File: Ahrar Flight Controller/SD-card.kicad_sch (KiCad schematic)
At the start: 16 parts, among them J4 1040310811

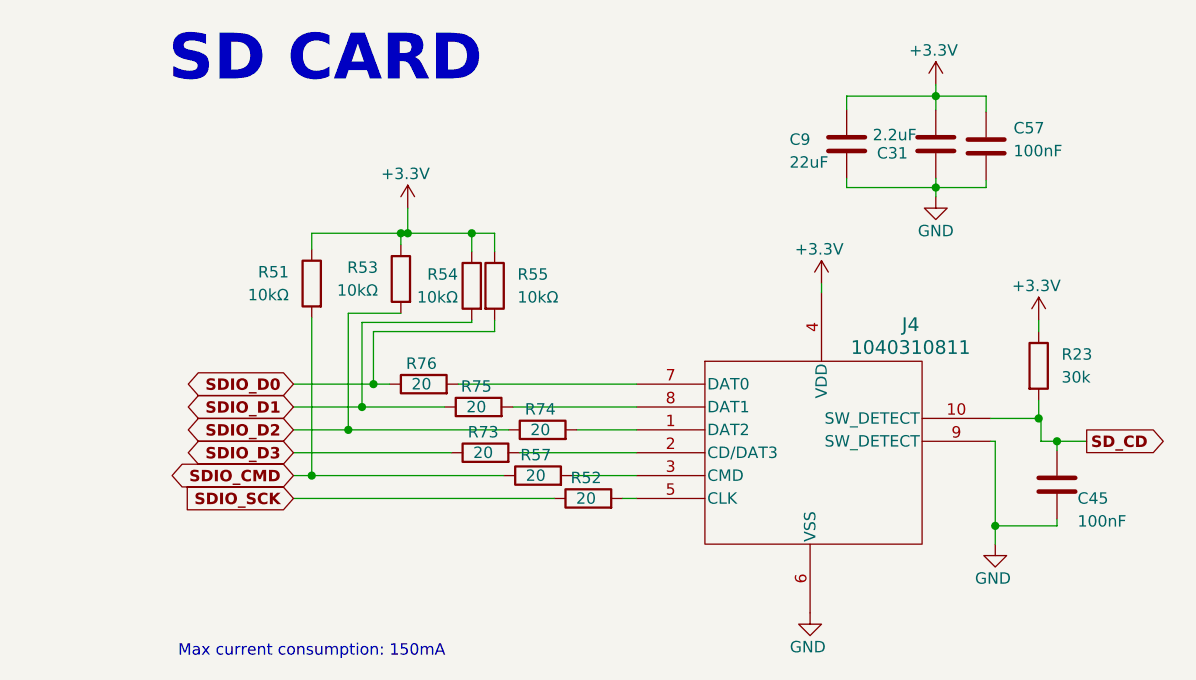
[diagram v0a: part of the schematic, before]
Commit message: .
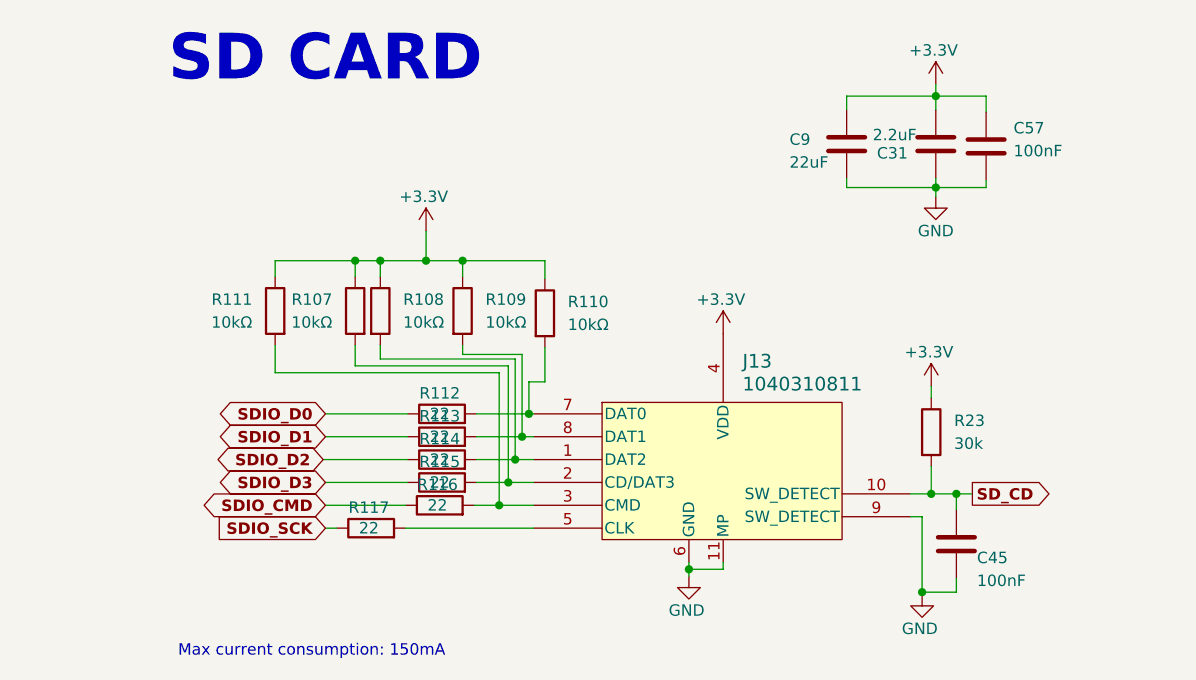
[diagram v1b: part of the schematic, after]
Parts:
- removed J4: 1040310811, Molex 1040310811:104031-0811_MOL, symbol 2026-07-10_16-12-29:1040310811
- removed R51, R53, R54, R55: 10kΩ, Resistor_SMD:R_0402_1005Metric, symbol Device:R
- removed R52, R57, R73, R74, R75, R76: 20, Resistor_SMD:R_0402_1005Metric, symbol Device:R
- added J13: 1040310811, Molex 1040310811:104031-0811_MOL, symbol 2026-07-10_16-12-29:1040310811
- added R107, R108, R109, R110, R111: 10kΩ, Resistor_SMD:R_0402_1005Metric, symbol Device:R
- added R112, R113, R114, R115, R116, R117: 22, Resistor_SMD:R_0402_1005Metric, symbol Device:R
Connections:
- net +3.3V: now also J13.4 (VDD), R107.1, R108.1, R109.1, R110.1, R111.1
- net GND: now also J13.11 (MP), J13.12 (MP), J13.13 (MP), J13.14 (MP), J13.6 (GND), J13.9 (SW_DETECT)
- net SDIO_CMD: now also R116.1
- net SDIO_D0: now also R112.1
- net SDIO_D1: now also R113.1
- net SDIO_D2: now also R114.1
- net SDIO_D3: now also R115.1
- net SDIO_SCK: now also R117.1
- net SD_CD: now also J13.10 (SW_DETECT)
- new net: J13.7 (DAT0), R110.2, R112.2
- new net: J13.1 (DAT2), R108.2, R114.2
- new net: J13.2 (CD/DAT3), R107.2, R115.2
- new net: J13.3 (CMD), R111.2, R116.2
- new net: J13.5 (CLK), R117.2
- new net: J13.8 (DAT1), R109.2, R113.2
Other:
- moved on the sheet: C45, R23
